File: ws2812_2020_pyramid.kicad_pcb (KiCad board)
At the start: 2 copper layers, 57.2 x 30.5 mm, 51 parts

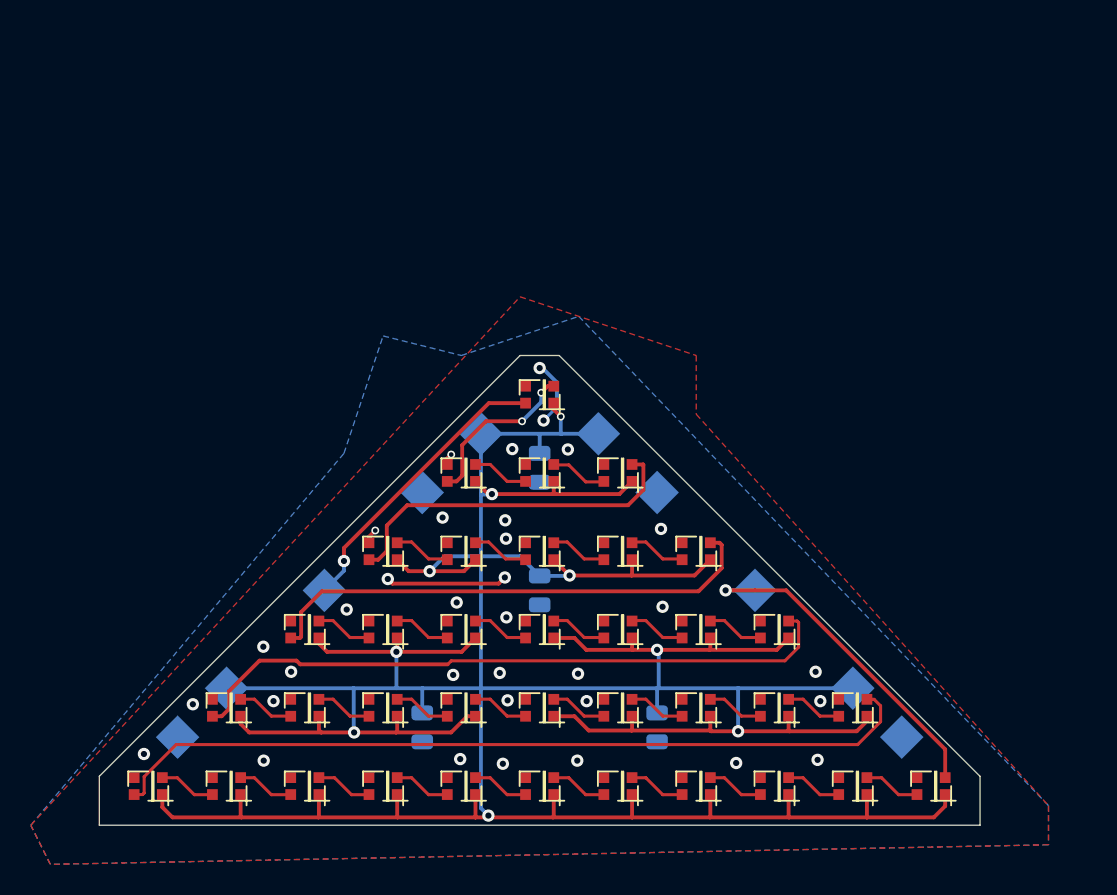
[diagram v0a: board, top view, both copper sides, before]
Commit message: Finish design
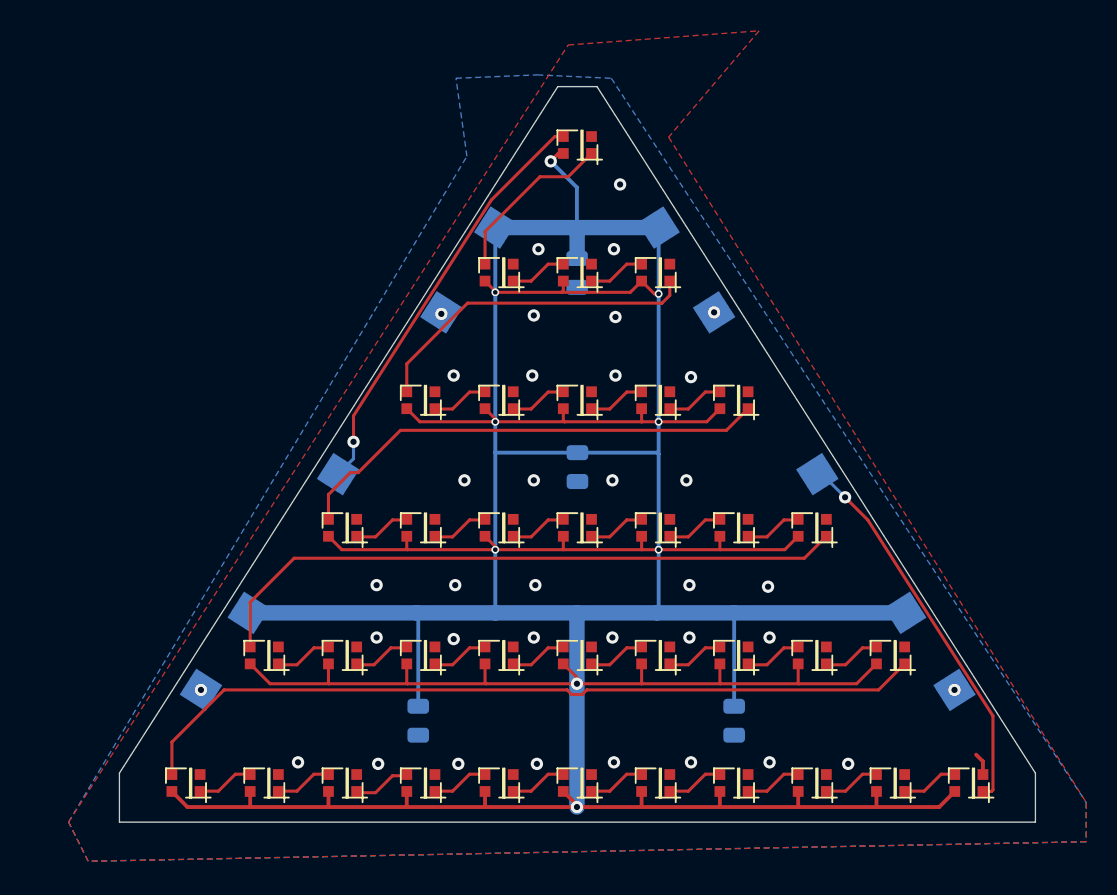
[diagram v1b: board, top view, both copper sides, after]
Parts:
- moved D1 16.4 mm to (121.8, 37.1)
- moved BR2 13.9 mm to (127.1, 42.5), turned to 122.5 degrees
- moved BR1 13.4 mm to (116.5, 42.5), turned to 237.5 degrees
- moved D2 13.2 mm to (116.8, 45.4)
- moved D3 13.2 mm to (121.8, 45.4)
- moved D4 13.2 mm to (126.9, 45.4)
- moved C1 12.9 mm to (121.8, 45.4)
- moved BR4 12.3 mm to (130.7, 48.0), turned to 122.5 degrees
- moved BR3 11.8 mm to (113.0, 48.0), turned to 237.5 degrees
- moved D9 10.1 mm to (132.0, 53.7)
- moved D5 10.1 mm to (111.7, 53.7)
- moved D6 10.1 mm to (116.8, 53.7)
- moved D7 10.1 mm to (121.8, 53.7)
- moved D8 10.1 mm to (126.9, 53.7)
- moved BR6 8.56 mm to (137.4, 58.5), turned to 122.5 degrees
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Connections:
- D1 pad 1: +5V -> Net-(D1-Pad1)
- D1 pad 2: Net-(D1-Pad2) -> GND
- D1 pad 3: GND -> DIN
- D1 pad 4: DIN -> +5V
- D10 pad 1: +5V -> Net-(D10-Pad1)
- D10 pad 2: Net-(D10-Pad2) -> GND
- D10 pad 3: GND -> Net-(D10-Pad3)
- D10 pad 4: Net-(D10-Pad4) -> +5V
- D11 pad 1: +5V -> Net-(D11-Pad1)
- D11 pad 2: Net-(D11-Pad2) -> GND
- D11 pad 3: GND -> Net-(D10-Pad1)
- D11 pad 4: Net-(D10-Pad2) -> +5V
- D12 pad 1: +5V -> Net-(D12-Pad1)
- D12 pad 2: Net-(D12-Pad2) -> GND
- D12 pad 3: GND -> Net-(D11-Pad1)
- D12 pad 4: Net-(D11-Pad2) -> +5V
- D13 pad 1: +5V -> Net-(D13-Pad1)
- D13 pad 2: Net-(D13-Pad2) -> GND
- D13 pad 3: GND -> Net-(D12-Pad1)
- D13 pad 4: Net-(D12-Pad2) -> +5V
- D14 pad 1: +5V -> Net-(D14-Pad1)
- D14 pad 2: Net-(D14-Pad2) -> GND
- D14 pad 3: GND -> Net-(D13-Pad1)
- D14 pad 4: Net-(D13-Pad2) -> +5V
- D15 pad 1: +5V -> Net-(D15-Pad1)
- D15 pad 2: Net-(D15-Pad2) -> GND
- D15 pad 3: GND -> Net-(D14-Pad1)
- D15 pad 4: Net-(D14-Pad2) -> +5V
- D16 pad 1: +5V -> Net-(D16-Pad1)
- D16 pad 2: Net-(D16-Pad2) -> GND
- D16 pad 3: GND -> Net-(D15-Pad1)
- D16 pad 4: Net-(D15-Pad2) -> +5V
- D17 pad 1: +5V -> Net-(D17-Pad1)
- D17 pad 2: Net-(D17-Pad2) -> GND
- D17 pad 3: GND -> Net-(D16-Pad1)
- D17 pad 4: Net-(D16-Pad2) -> +5V
- D18 pad 1: +5V -> Net-(D18-Pad1)
- D18 pad 2: Net-(D18-Pad2) -> GND
- D18 pad 3: GND -> Net-(D17-Pad1)
- D18 pad 4: Net-(D17-Pad2) -> +5V
- D19 pad 1: +5V -> Net-(D19-Pad1)
- D19 pad 2: Net-(D19-Pad2) -> GND
- D19 pad 3: GND -> Net-(D18-Pad1)
- D19 pad 4: Net-(D18-Pad2) -> +5V
- D2 pad 1: +5V -> Net-(D2-Pad1)
- D2 pad 2: Net-(D2-Pad2) -> GND
- D2 pad 3: GND -> Net-(D1-Pad1)
- D2 pad 4: Net-(D1-Pad2) -> +5V
- D20 pad 1: +5V -> Net-(D20-Pad1)
- D20 pad 2: Net-(D20-Pad2) -> GND
- D20 pad 3: GND -> Net-(D19-Pad1)
- D20 pad 4: Net-(D19-Pad2) -> +5V
- D21 pad 1: +5V -> Net-(D21-Pad1)
- D21 pad 2: Net-(D21-Pad2) -> GND
- D21 pad 3: GND -> Net-(D20-Pad1)
- D21 pad 4: Net-(D20-Pad2) -> +5V
- D22 pad 1: +5V -> Net-(D22-Pad1)
- D22 pad 2: Net-(D22-Pad2) -> GND
- D22 pad 3: GND -> Net-(D21-Pad1)
- D22 pad 4: Net-(D21-Pad2) -> +5V
- D23 pad 1: +5V -> Net-(D23-Pad1)
- D23 pad 2: Net-(D23-Pad2) -> GND
- D23 pad 3: GND -> Net-(D22-Pad1)
- D23 pad 4: Net-(D22-Pad2) -> +5V
- D24 pad 1: +5V -> Net-(D24-Pad1)
- D24 pad 2: Net-(D24-Pad2) -> GND
- D24 pad 3: GND -> Net-(D23-Pad1)
- D24 pad 4: Net-(D23-Pad2) -> +5V
- D25 pad 1: +5V -> Net-(D25-Pad1)
- D25 pad 2: Net-(D25-Pad2) -> GND
- D25 pad 3: GND -> Net-(D24-Pad1)
- D25 pad 4: Net-(D24-Pad2) -> +5V
- D26 pad 1: +5V -> Net-(D26-Pad1)
- D26 pad 2: Net-(D26-Pad2) -> GND
- D26 pad 3: GND -> Net-(D25-Pad1)
- D26 pad 4: Net-(D25-Pad2) -> +5V
- D27 pad 1: +5V -> Net-(D27-Pad1)
- D27 pad 2: Net-(D27-Pad2) -> GND
- D27 pad 3: GND -> Net-(D26-Pad1)
- D27 pad 4: Net-(D26-Pad2) -> +5V
- D28 pad 1: +5V -> Net-(D28-Pad1)
- D28 pad 2: Net-(D28-Pad2) -> GND
- D28 pad 3: GND -> Net-(D27-Pad1)
- D28 pad 4: Net-(D27-Pad2) -> +5V
- D29 pad 1: +5V -> Net-(D29-Pad1)
- D29 pad 2: Net-(D29-Pad2) -> GND
- D29 pad 3: GND -> Net-(D28-Pad1)
- D29 pad 4: Net-(D28-Pad2) -> +5V
- D3 pad 1: +5V -> Net-(D3-Pad1)
- D3 pad 2: Net-(D3-Pad2) -> GND
- D3 pad 3: GND -> Net-(D2-Pad1)
- D3 pad 4: Net-(D2-Pad2) -> +5V
- D30 pad 1: +5V -> Net-(D30-Pad1)
- D30 pad 2: Net-(D30-Pad2) -> GND
- D30 pad 3: GND -> Net-(D29-Pad1)
- D30 pad 4: Net-(D29-Pad2) -> +5V
- D31 pad 1: +5V -> Net-(D31-Pad1)
- D31 pad 2: Net-(D31-Pad2) -> GND
- D31 pad 3: GND -> Net-(D30-Pad1)
- D31 pad 4: Net-(D30-Pad2) -> +5V
- D32 pad 1: +5V -> Net-(D32-Pad1)
- D32 pad 2: Net-(D32-Pad2) -> GND
- D32 pad 3: GND -> Net-(D31-Pad1)
- D32 pad 4: Net-(D31-Pad2) -> +5V
- D33 pad 1: +5V -> Net-(D33-Pad1)
- D33 pad 2: Net-(D33-Pad2) -> GND
- D33 pad 3: GND -> Net-(D32-Pad1)
- D33 pad 4: Net-(D32-Pad2) -> +5V
- D34 pad 1: +5V -> Net-(D34-Pad1)
- D34 pad 2: Net-(D34-Pad2) -> GND
- D34 pad 3: GND -> Net-(D33-Pad1)
- D34 pad 4: Net-(D33-Pad2) -> +5V
- D35 pad 1: +5V -> Net-(D35-Pad1)
- D35 pad 2: Net-(D35-Pad2) -> GND
- D35 pad 3: GND -> Net-(D34-Pad1)
- D35 pad 4: Net-(D34-Pad2) -> +5V
- D36 pad 1: +5V -> DOUT
- D36 pad 2: DOUT -> GND
- D36 pad 3: GND -> Net-(D35-Pad1)
- D36 pad 4: Net-(D35-Pad2) -> +5V
- D4 pad 1: +5V -> Net-(D4-Pad1)
- D4 pad 2: Net-(D4-Pad2) -> GND
- D4 pad 3: GND -> Net-(D3-Pad1)
- D4 pad 4: Net-(D3-Pad2) -> +5V
- D5 pad 1: +5V -> Net-(D5-Pad1)
- D5 pad 2: Net-(D5-Pad2) -> GND
- D5 pad 3: GND -> Net-(D4-Pad1)
- D5 pad 4: Net-(D4-Pad2) -> +5V
- D6 pad 1: +5V -> Net-(D6-Pad1)
- D6 pad 2: Net-(D6-Pad2) -> GND
- D6 pad 3: GND -> Net-(D5-Pad1)
- D6 pad 4: Net-(D5-Pad2) -> +5V
- D7 pad 1: +5V -> Net-(D7-Pad1)
- D7 pad 2: Net-(D7-Pad2) -> GND
- D7 pad 3: GND -> Net-(D6-Pad1)
- D7 pad 4: Net-(D6-Pad2) -> +5V
- D8 pad 1: +5V -> Net-(D8-Pad1)
- D8 pad 2: Net-(D8-Pad2) -> GND
- D8 pad 3: GND -> Net-(D7-Pad1)
- D8 pad 4: Net-(D7-Pad2) -> +5V
- D9 pad 1: +5V -> Net-(D10-Pad3)
- D9 pad 2: Net-(D10-Pad4) -> GND
- D9 pad 3: GND -> Net-(D8-Pad1)
- D9 pad 4: Net-(D8-Pad2) -> +5V
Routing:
- net +5V: track 269.3 -> 331.8 mm
- net Net-(D25-Pad2): track 53.4 -> 0.00 mm
- net Net-(D25-Pad1): track 0.00 -> 52.0 mm
- net Net-(D16-Pad2): track 43.1 -> 0.00 mm
- net Net-(D16-Pad1): track 0.00 -> 42.1 mm
- net Net-(D10-Pad4): track 33.1 -> 0.00 mm
- net Net-(D10-Pad3): track 0.00 -> 31.1 mm
- net Net-(D4-Pad2): track 23.0 -> 0.00 mm
- net Net-(D4-Pad1): track 0.00 -> 21.6 mm
- net GND: track 14.0 -> 1.47 mm, vias 34 -> 36
- net Net-(D1-Pad1): track 0.00 -> 11.1 mm
- net Net-(D1-Pad2): track 11.0 -> 0.00 mm, vias 2 -> 0
- net DIN: track 19.0 -> 27.2 mm
- net Net-(D22-Pad1): track 0.00 -> 3.71 mm
- net Net-(D8-Pad1): track 0.00 -> 3.71 mm
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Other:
- board size 57.2 x 30.5 mm -> 59.4 x 47.7 mm
- board text added: "v0.0.1 11/09/20"
- board text removed: "v0.0.0 10/30/20"
